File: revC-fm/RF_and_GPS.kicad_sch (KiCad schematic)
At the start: 38 parts, among them J2 SMPM-PS-P-HG-ST-EM-1, J3 SMPM-PS-P-HG-ST-EM-1, J4 SMPM-PS-P-HG-ST-EM-1, Q5 BSZ180P03NS3GATMA1, U21 RFM98PW, U22 RFM9xBreakout, U23 ORION B16, U24 RFM98PW, U25 RFM9xBreakout

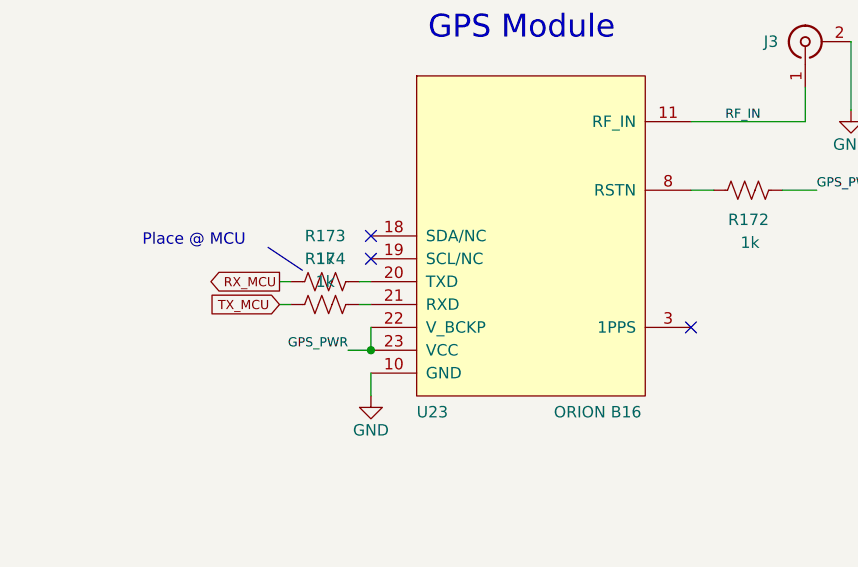
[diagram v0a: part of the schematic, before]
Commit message: fm layout
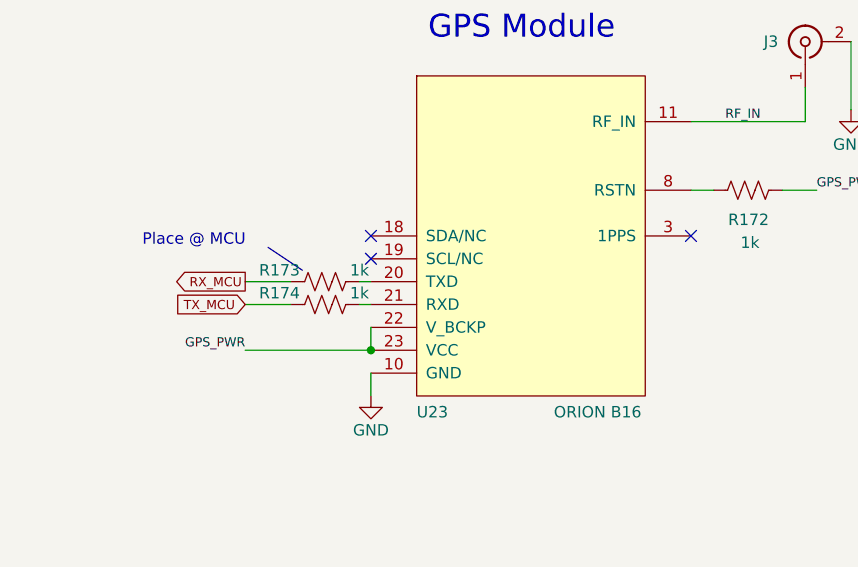
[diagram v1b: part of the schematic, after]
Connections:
- now unconnected: U23.1 (NC), U23.14 (NC), U23.15 (NC), U23.16 (NC), U23.17 (NC), U23.2 (NC), U23.4 (NC), U23.5 (NC), U23.6 (NC), U23.7 (NC), U23.9 (NC)
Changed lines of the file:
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@@
   (no_connect (at 95.25 90.17))
   (no_connect (at 99.06 62.23))
-  (no_connect (at 254 125.73))
+  (no_connect (at 254 115.57))
   (no_connect (at 93.98 176.53))
   (no_connect (at 99.06 57.15))
@@
     (stroke (width 0) (type default))
   )
-  (wire (pts (xy 209.55 120.65) (xy 208.28 120.65))
+  (wire (pts (xy 209.55 120.65) (xy 204.47 120.65))
     (stroke (width 0) (type default))
   )
@@
     (stroke (width 0) (type default))
   )
-  (wire (pts (xy 218.44 128.27) (xy 215.9 128.27))
+  (wire (pts (xy 218.44 128.27) (xy 204.47 128.27))
     (stroke (width 0) (type default))
   )
@@
     (stroke (width 0) (type default))
   )
-  (wire (pts (xy 209.55 123.19) (xy 208.28 123.19))
+  (wire (pts (xy 209.55 123.19) (xy 204.47 123.19))
     (stroke (width 0) (type default))
   )
@@
     (effects (font (size 1.016 1.016)) (justify left bottom))
   )
-  (label "GPS_PWR" (at 215.9 128.27 180) (fields_autoplaced)
+  (label "GPS_PWR" (at 204.47 128.27 180) (fields_autoplaced)
     (effects (font (size 1.016 1.016)) (justify right bottom))
   )
@@
     )
   )
-  (global_label "TX_MCU" (shape input) (at 208.28 123.19 180) (fields_autoplaced)
-    (effects (font (size 1.016 1.016)) (justify right))
-    (property "Intersheetrefs" "${INTERSHEET_REFS}" (at 200.7214 123.19 0)
+  (global_label "TX_MCU" (shape input) (at 204.47 123.19 180) (fields_autoplaced)
+    (effects (font (size 1.016 1.016)) (justify right))
+    (property "Intersheetrefs" "${INTERSHEET_REFS}" (at 196.9114 123.19 0)
       (effects (font (size 1.016 1.016)) (justify right) hide)
     )
@@
     )
   )
-  (global_label "RX_MCU" (shape output) (at 208.28 120.65 180) (fields_autoplaced)
-    (effects (font (size 1.016 1.016)) (justify right))
-    (property "Intersheetrefs" "${INTERSHEET_REFS}" (at 200.4795 120.65 0)
+  (global_label "RX_MCU" (shape output) (at 204.47 120.65 180) (fields_autoplaced)
+    (effects (font (size 1.016 1.016)) (justify right))
+    (property "Intersheetrefs" "${INTERSHEET_REFS}" (at 196.6695 120.65 0)
       (effects (font (size 1.016 1.016)) (justify right) hide)
     )
@@
   )
   (symbol (lib_id "Device:R_US") (at 213.36 120.65 90) (unit 1)
-    (in_bom yes) (on_board yes) (dnp no) (fields_autoplaced)
-    (property "Reference" "R173" (at 213.36 115.57 90)
-      (effects (font (size 1.27 1.27)))
-    )
-    (property "Value" "1k" (at 213.36 118.11 90)
+    (in_bom yes) (on_board yes) (dnp no)
+    (property "Reference" "R173" (at 208.28 119.38 90)
+      (effects (font (size 1.27 1.27)))
+    )
+    (property "Value" "1k" (at 217.17 119.38 90)
       (effects (font (size 1.27 1.27)))
     )
@@
   )
   (symbol (lib_id "Device:R_US") (at 213.36 123.19 90) (unit 1)
-    (in_bom yes) (on_board yes) (dnp no) (fields_autoplaced)
-    (property "Reference" "R174" (at 213.36 118.11 90)
-      (effects (font (size 1.27 1.27)))
-    )
-    (property "Value" "1k" (at 213.36 120.65 90)
-      (effects (font (size 1.27 1.27)))
-    )
+    (in_bom yes) (on_board yes) (dnp no)
+    (property "Reference" "R174" (at 208.28 121.92 90)
+      (effects (font (size 1.27 1.27)))
+    )
+    (property "Value" "1k" (at 217.17 121.92 90)
+      (effects (font (size 1.27 1.27)))
+    )
